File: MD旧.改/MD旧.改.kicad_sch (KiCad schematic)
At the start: 42 parts, among them J1 Conn_01x04_Pin, J2 Conn_02x04_Odd_Even, J3 XT60-M, J4 XT60-M

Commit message: 詰め詰め
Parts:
- R11: footprint Resistor_THT:R_Axial_DIN0207_L6.3mm_D2.5mm_P10.16mm_Horizontal -> Library:R_Axial_DIN0207_L6.3mm_D2.5mm_P10.16mm_Horizontal_kai
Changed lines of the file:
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@@
 			)
 		)
-		(property "Footprint" "Resistor_THT:R_Axial_DIN0207_L6.3mm_D2.5mm_P10.16mm_Horizontal"
+		(property "Footprint" "Library:R_Axial_DIN0207_L6.3mm_D2.5mm_P10.16mm_Horizontal_kai"
 			(at 207.772 130.81 90)
 			(effects

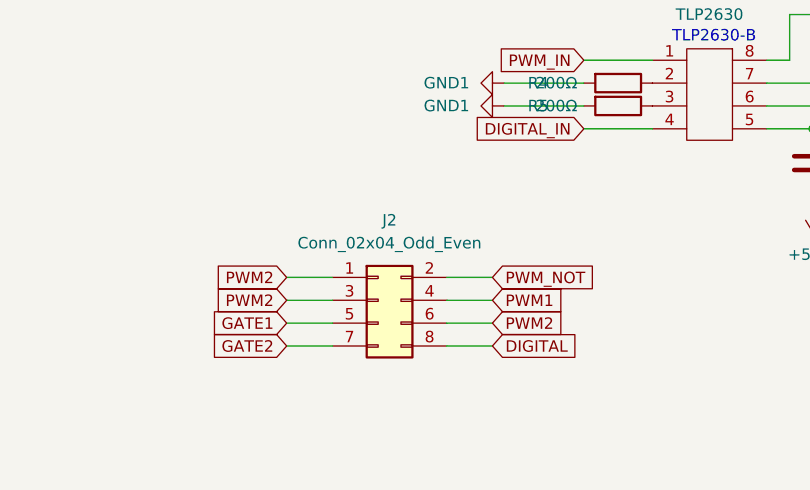
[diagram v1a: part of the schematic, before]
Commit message: あ
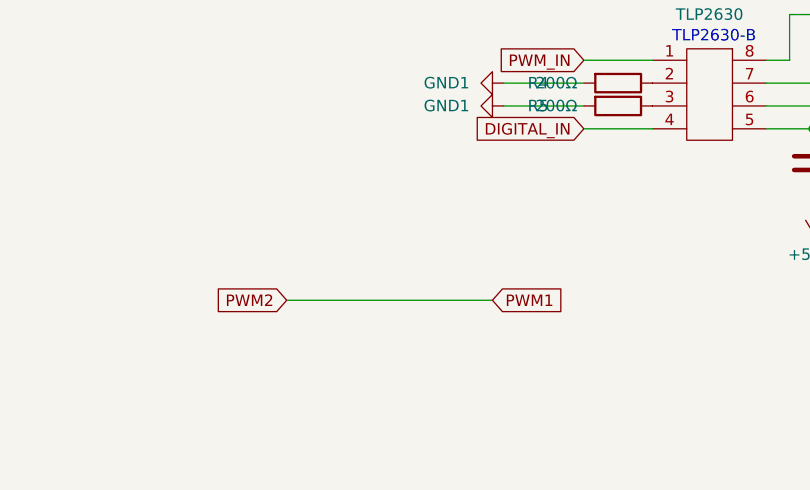
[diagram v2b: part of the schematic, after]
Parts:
- removed J2: Conn_02x04_Odd_Even, Connector_PinHeader_2.54mm:PinHeader_2x04_P2.54mm_Vertical, symbol Connector_Generic:Conn_02x04_Odd_Even
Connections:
- net PWM2 is gone; now on net PWM1: IC2_AND1.1, IC2_AND1.4
